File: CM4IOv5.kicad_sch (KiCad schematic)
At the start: 12 parts, among them J15 HTST-110-X-X-D-RA, SW1 1301.9314.24

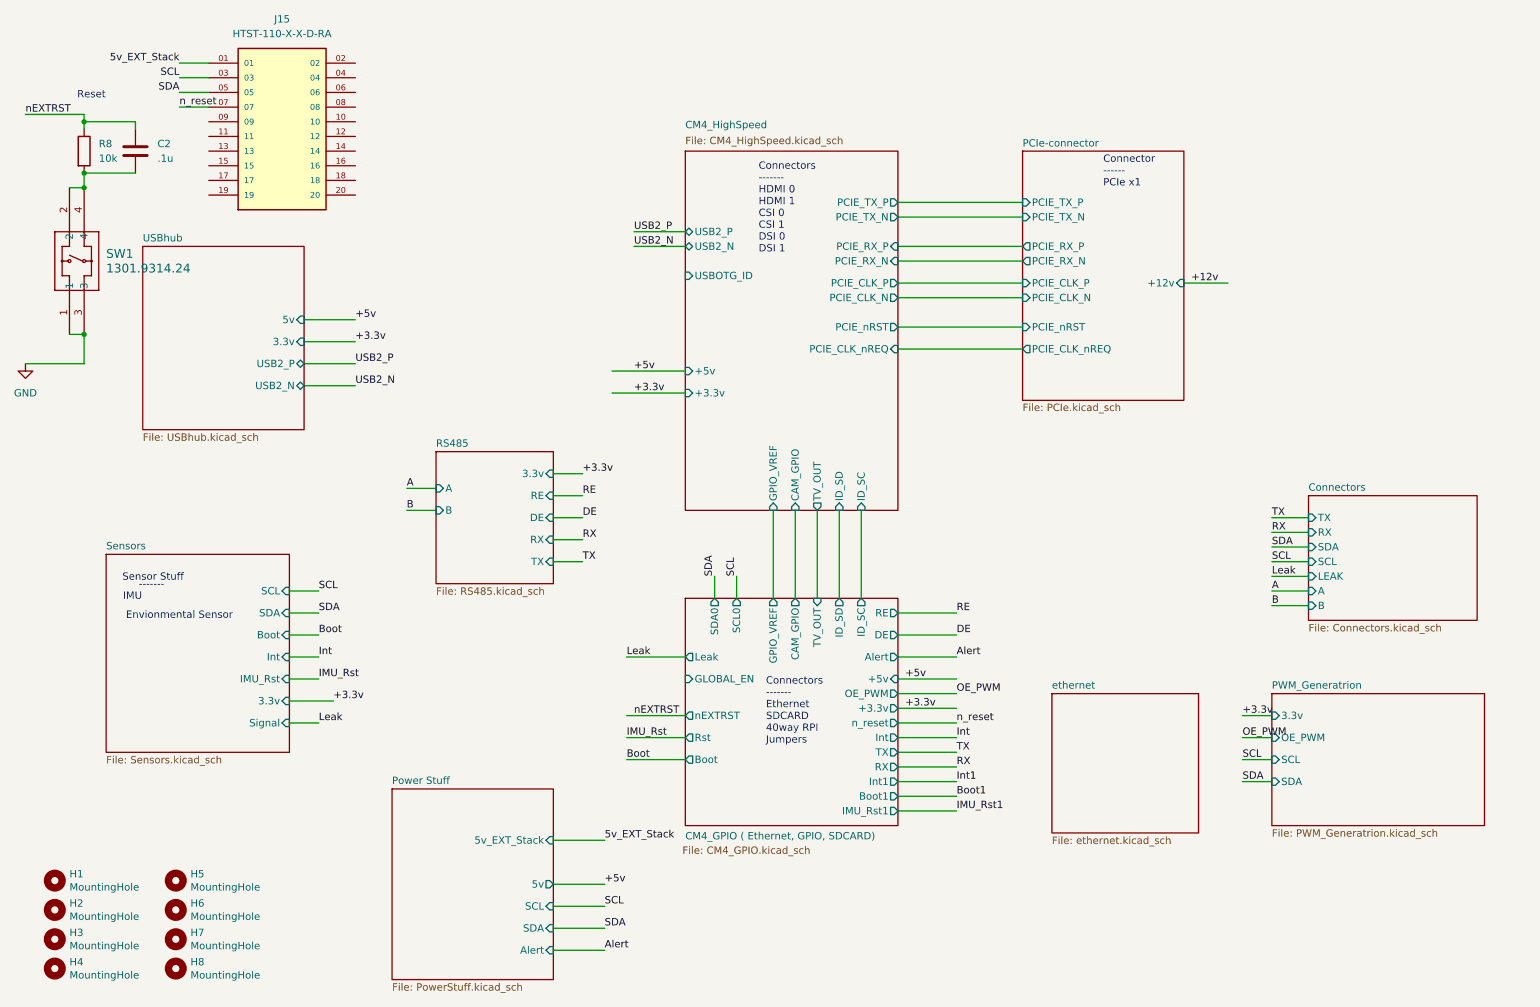
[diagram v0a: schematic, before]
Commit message: stuff
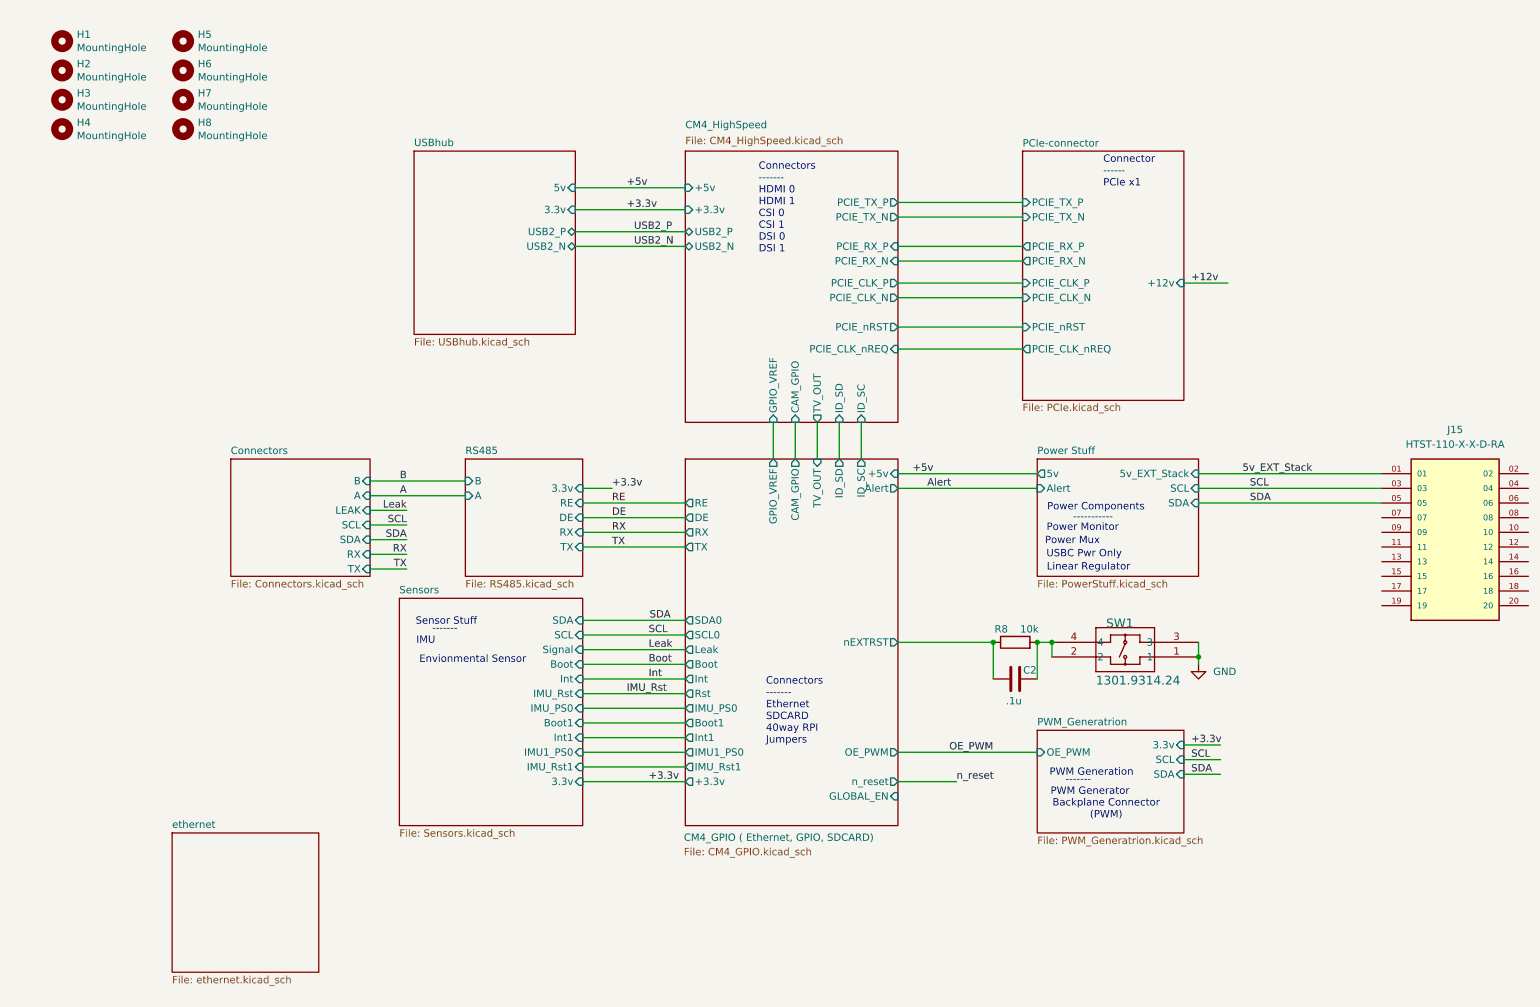
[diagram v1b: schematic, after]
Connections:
- net n_reset: no longer J15.07
- net nEXTRST renamed CM4_GPIO ( Ethernet, GPIO, SDCARD)/nEXTRST
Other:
- sheet CM4_GPIO ( Ethernet, GPIO, SDCARD) ports: added IMU1_PS0, IMU_PS0; removed none
- sheet CM4_HighSpeed ports: added none; removed USBOTG_ID
- sheet Sensors ports: added Boot1, IMU1_PS0, IMU_PS0, IMU_Rst1, Int1; removed none
- note added: "-----------"
- note added: "Backplane Connector (PWM)"
- note added: "Linear Regulator"
- note added: "PWM Generation"
- note added: "PWM Generator"
- note added: "Power Components"
- note added: "Power Monitor"
- note added: "Power Mux"
- note added: "USBC Pwr Only"
- note removed: "Reset"
- moved on the sheet: H1, H2, H3, H4, H5, H6, H7, H8, J15, R8, SW1
